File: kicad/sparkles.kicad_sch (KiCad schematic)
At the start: 70 parts

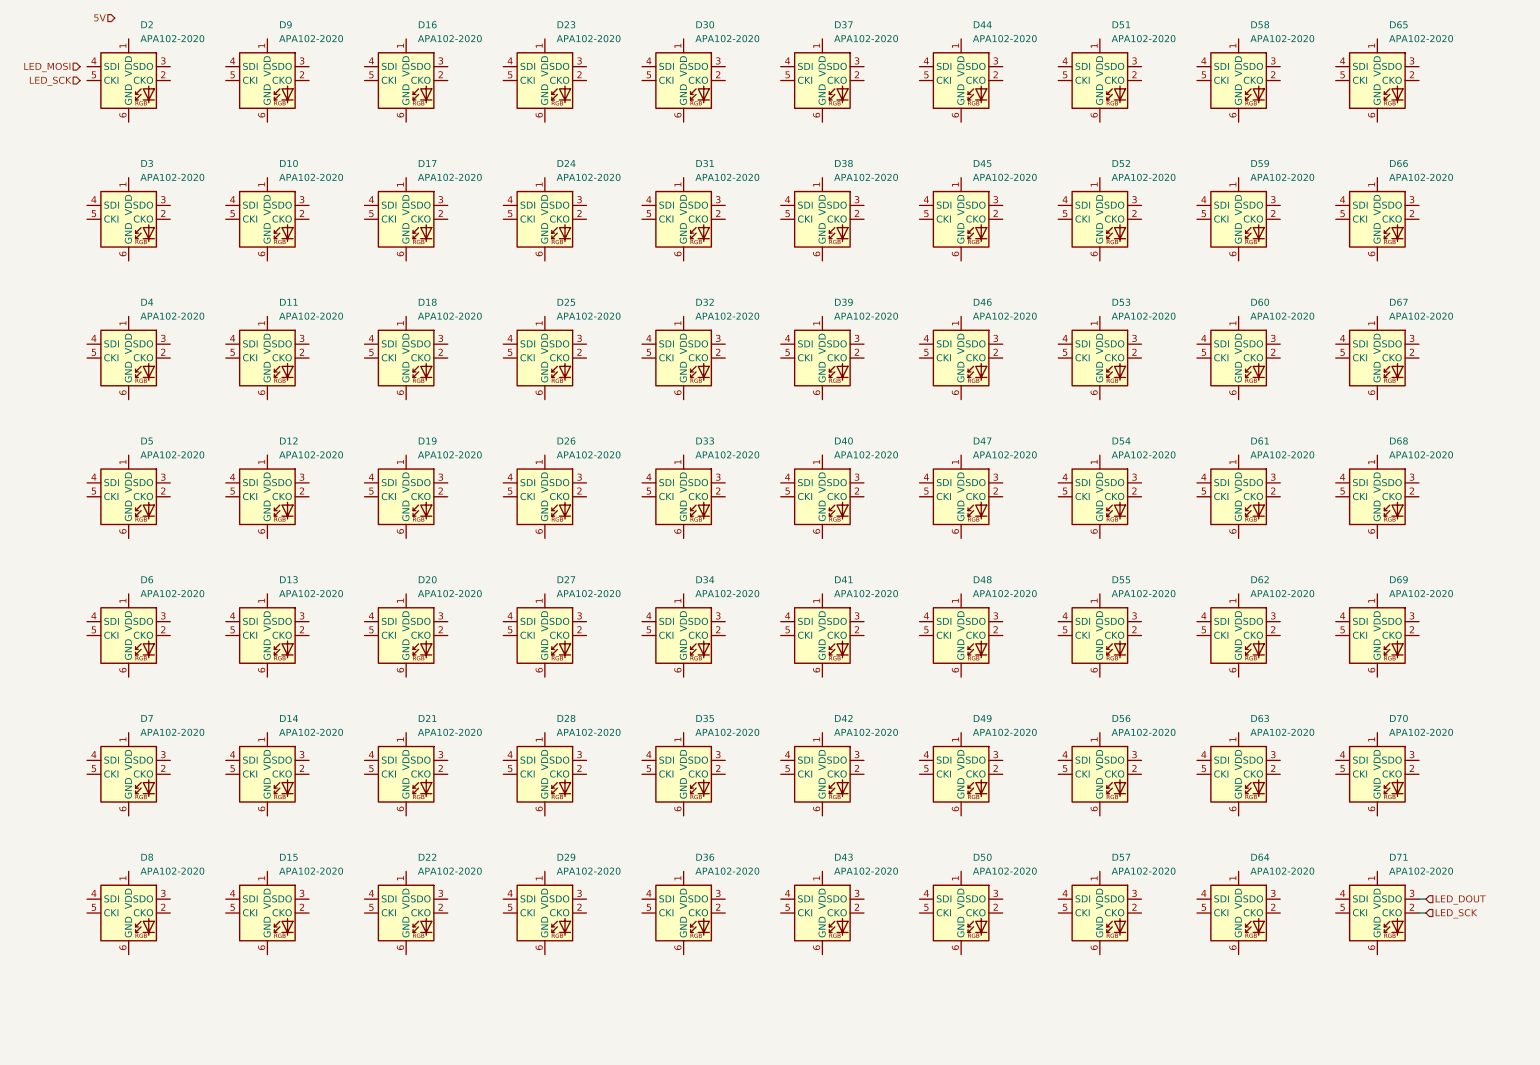
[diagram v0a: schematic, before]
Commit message: updates
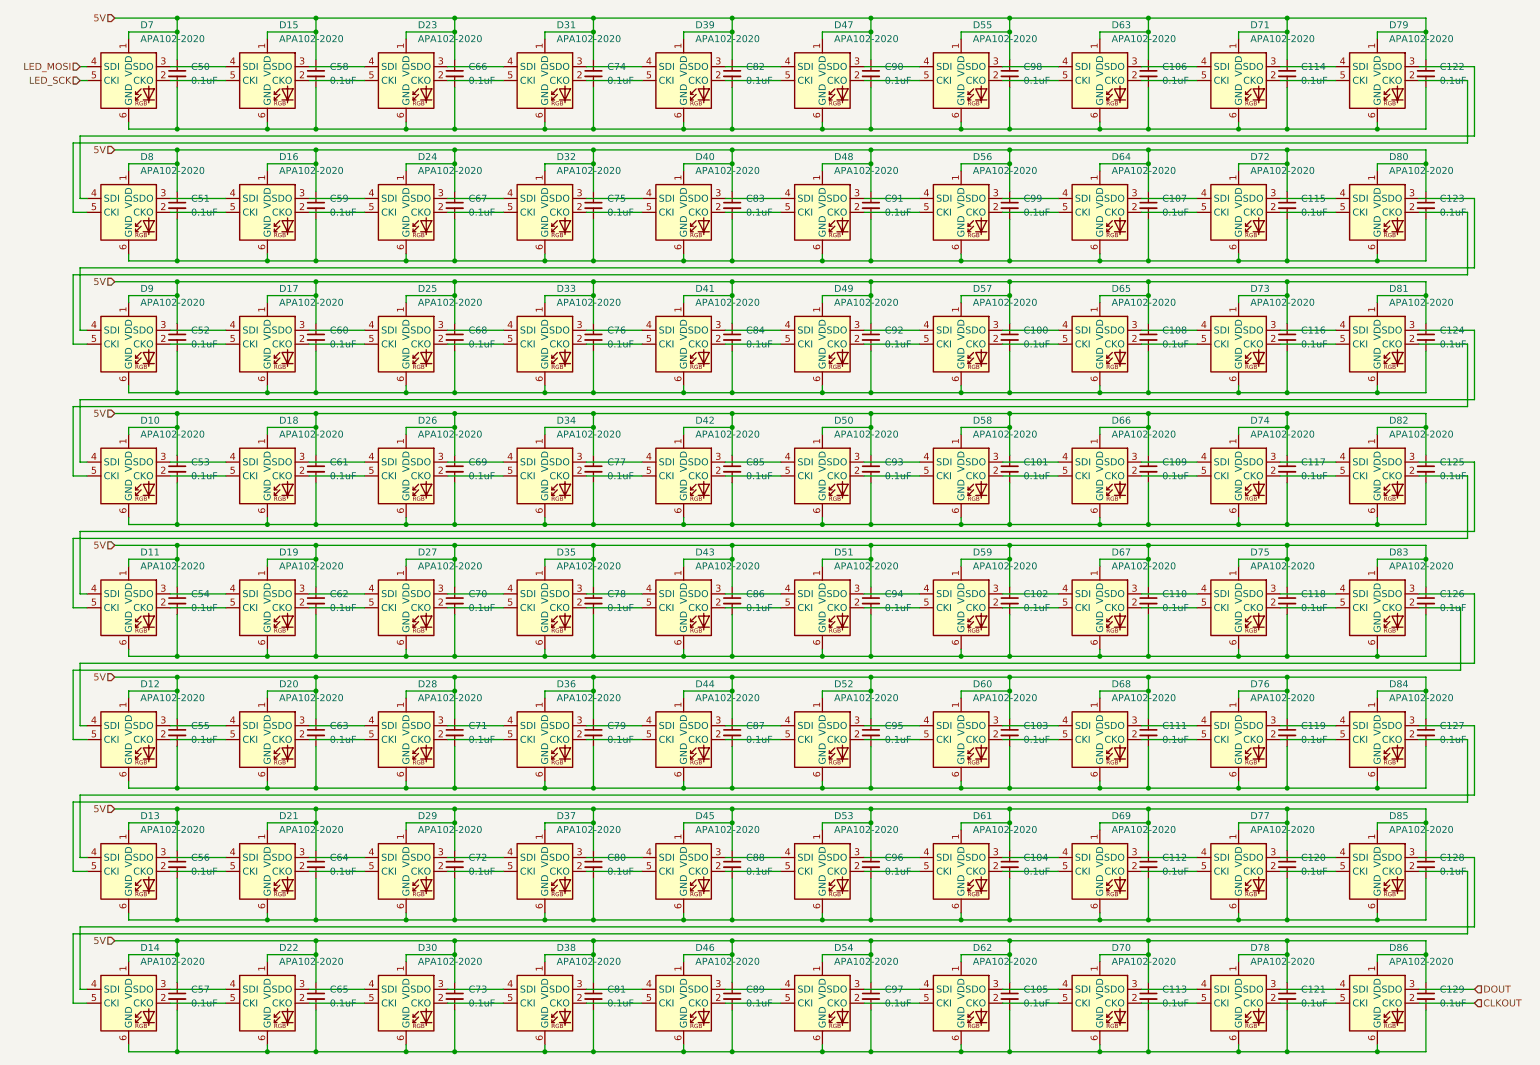
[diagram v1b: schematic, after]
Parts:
- removed D15, D3, D31, D39, D4, D47, D5, D55, D6, D63, D7, D71: APA102-2020, LED_SMD:LED-APA102-2020, symbol LED:APA102-2020
- added C100, C101, C102, C103, C104, C105, C106, C107, C108, C109, C110, C111, C112, C113, C114, C115, C116, C117, C118, C119, C120, C121, C122, C123, C124, C125, C126, C127, C128, C129, C50, C51, C52, C53, C54, C55, C56, C57, C58, C59, C60, C61, C62, C63, C64, C65, C66, C67, C68, C69, C70, C71, C72, C73, C74, C75, C76, C77, C78, C79, C80, C81, C82, C83, C84, C85, C86, C87, C88, C89, C90, C91, C92, C93, C94, C95, C96, C97, C98, C99: 0.1uF, symbol Device:C_Small
- added D16, D30, D37, D44, D51, D58, D65, D72, D73, D74, D75, D76, D77, D78, D80, D81, D82, D83, D84, D85, D86, D9: APA102-2020, LED_SMD:LED-APA102-2020, symbol LED:APA102-2020
- renumbered D9 to D15, D16 to D23, D23 to D31, D30 to D39, D37 to D47, D44 to D55, D51 to D63, D2 to D7, D58 to D71, D65 to D79
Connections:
- net 5V: now also D10.1 (VDD), D11.1 (VDD), D12.1 (VDD), D13.1 (VDD), D14.1 (VDD), D15.1 (VDD), D17.1 (VDD), D18.1 (VDD), D19.1 (VDD), D20.1 (VDD), D21.1 (VDD), D22.1 (VDD), D23.1 (VDD), D24.1 (VDD), D25.1 (VDD), D26.1 (VDD), D27.1 (VDD), D28.1 (VDD), D29.1 (VDD), D31.1 (VDD), D32.1 (VDD), D33.1 (VDD), D34.1 (VDD), D35.1 (VDD), D36.1 (VDD), D38.1 (VDD), D39.1 (VDD), D40.1 (VDD), D41.1 (VDD), D42.1 (VDD), D43.1 (VDD), D45.1 (VDD), D46.1 (VDD), D47.1 (VDD), D48.1 (VDD), D49.1 (VDD), D50.1 (VDD), D52.1 (VDD), D53.1 (VDD), D54.1 (VDD), D55.1 (VDD), D56.1 (VDD), D57.1 (VDD), D59.1 (VDD), D60.1 (VDD), D61.1 (VDD), D62.1 (VDD), D63.1 (VDD), D64.1 (VDD), D66.1 (VDD), D67.1 (VDD), D68.1 (VDD), D69.1 (VDD), D7.1 (VDD), D70.1 (VDD), D71.1 (VDD), D79.1 (VDD), D8.1 (VDD), C100.1, C101.1, C102.1, C103.1, C104.1, C105.1, C106.1, C107.1, C108.1, C109.1, C110.1, C111.1, C112.1, C113.1, C114.1, C115.1, C116.1, C117.1, C118.1, C119.1, C120.1, C121.1, C122.1, C123.1, C124.1, C125.1, C126.1, C127.1, C128.1, C129.1, C50.1, C51.1, C52.1, C53.1, C54.1, C55.1, C56.1, C57.1, C58.1, C59.1, C60.1, C61.1, C62.1, C63.1, C64.1, C65.1, C66.1, C67.1, C68.1, C69.1, C70.1, C71.1, C72.1, C73.1, C74.1, C75.1, C76.1, C77.1, C78.1, C79.1, C80.1, C81.1, C82.1, C83.1, C84.1, C85.1, C86.1, C87.1, C88.1, C89.1, C90.1, C91.1, C92.1, C93.1, C94.1, C95.1, C96.1, C97.1, C98.1, C99.1, D16.1 (VDD), D30.1 (VDD), D37.1 (VDD), D44.1 (VDD), D51.1 (VDD), D58.1 (VDD), D65.1 (VDD), D72.1 (VDD), D73.1 (VDD), D74.1 (VDD), D75.1 (VDD), D76.1 (VDD), D77.1 (VDD), D78.1 (VDD), D80.1 (VDD), D81.1 (VDD), D82.1 (VDD), D83.1 (VDD), D84.1 (VDD), D85.1 (VDD), D86.1 (VDD), D9.1 (VDD)
- net LED_MOSI: now also D7.4 (SDI)
- net LED_SCK: now also D7.5 (CKI)
- net at D32.2 (CKO): now also D40.5 (CKI)
- net at D32.3 (SDO): now also D40.4 (SDI)
- net at D32.4 (SDI): now also D24.3 (SDO)
- net at D32.5 (CKI): now also D24.2 (CKO)
- net at D32.6 (GND): now also D24.6 (GND), D40.6 (GND), D48.6 (GND), D56.6 (GND), D64.6 (GND), D8.6 (GND), C107.2, C115.2, C123.2, C51.2, C59.2, C67.2, C75.2, C83.2, C91.2, C99.2, D16.6 (GND), D72.6 (GND), D80.6 (GND)
- net at D21.2 (CKO): now also D29.5 (CKI)
- net at D21.3 (SDO): now also D29.4 (SDI)
- net at D21.4 (SDI): now also D13.3 (SDO)
- net at D21.5 (CKI): now also D13.2 (CKO)
- net at D21.6 (GND): now also D13.6 (GND), D29.6 (GND), D45.6 (GND), D53.6 (GND), D61.6 (GND), D69.6 (GND), C104.2, C112.2, C120.2, C128.2, C56.2, C64.2, C72.2, C80.2, C88.2, C96.2, D37.6 (GND), D77.6 (GND), D85.6 (GND)
- net at D34.2 (CKO): now also D42.5 (CKI)
- net at D34.3 (SDO): now also D42.4 (SDI)
- net at D34.4 (SDI): now also D26.3 (SDO)
- net at D34.5 (CKI): now also D26.2 (CKO)
- net at D34.6 (GND): now also D10.6 (GND), D18.6 (GND), D26.6 (GND), D42.6 (GND), D50.6 (GND), D66.6 (GND), C101.2, C109.2, C117.2, C125.2, C53.2, C61.2, C69.2, C77.2, C85.2, C93.2, D58.6 (GND), D74.6 (GND), D82.6 (GND)
- net at D48.2 (CKO): now also D56.5 (CKI)
- net at D48.3 (SDO): now also D56.4 (SDI)
- net at D48.4 (SDI): now also D40.3 (SDO)
- net at D48.5 (CKI): now also D40.2 (CKO)
- net at D64.2 (CKO): now also D72.5 (CKI)
- net at D64.3 (SDO): now also D72.4 (SDI)
- net at D64.4 (SDI): now also D56.3 (SDO)
- net at D64.5 (CKI): now also D56.2 (CKO)
- net at D47.2 (CKO): now also D55.5 (CKI)
- net at D47.3 (SDO): now also D55.4 (SDI)
- net at D47.4 (SDI): now also D39.3 (SDO)
- net at D47.5 (CKI): now also D39.2 (CKO)
- net at D47.6 (GND): now also D15.6 (GND), D23.6 (GND), D31.6 (GND), D39.6 (GND), D55.6 (GND), D63.6 (GND), D7.6 (GND), D71.6 (GND), D79.6 (GND), C106.2, C114.2, C122.2, C50.2, C58.2, C66.2, C74.2, C82.2, C90.2, C98.2
- net at D39.4 (SDI): now also D31.3 (SDO)
- net at D39.5 (CKI): now also D31.2 (CKO)
- net at D36.2 (CKO): now also D44.5 (CKI)
- net at D36.3 (SDO): now also D44.4 (SDI)
- net at D36.4 (SDI): now also D28.3 (SDO)
- net at D36.5 (CKI): now also D28.2 (CKO)
- net at D36.6 (GND): now also D12.6 (GND), D20.6 (GND), D28.6 (GND), D52.6 (GND), D60.6 (GND), D68.6 (GND), C103.2, C111.2, C119.2, C127.2, C55.2, C63.2, C71.2, C79.2, C87.2, C95.2, D44.6 (GND), D76.6 (GND), D84.6 (GND)
- net at D11.2 (CKO): now also D19.5 (CKI)
- net at D11.3 (SDO): now also D19.4 (SDI)
- net at D11.4 (SDI): now also D82.3 (SDO)
- net at D11.5 (CKI): now also D82.2 (CKO)
- net at D11.6 (GND): now also D19.6 (GND), D27.6 (GND), D35.6 (GND), D43.6 (GND), D59.6 (GND), D67.6 (GND), C102.2, C110.2, C118.2, C126.2, C54.2, C62.2, C70.2, C78.2, C86.2, C94.2, D51.6 (GND), D75.6 (GND), D83.6 (GND)
- net at D38.2 (CKO): now also D46.5 (CKI)
- net at D38.3 (SDO): now also D46.4 (SDI)
- net at D38.4 (SDI): now also D30.3 (SDO)
- net at D38.5 (CKI): now also D30.2 (CKO)
- net at D38.6 (GND): now also D14.6 (GND), D22.6 (GND), D46.6 (GND), D54.6 (GND), D62.6 (GND), D70.6 (GND), C105.2, C113.2, C121.2, C129.2, C57.2, C65.2, C73.2, C81.2, C89.2, C97.2, D30.6 (GND), D78.6 (GND), D86.6 (GND)
- net at D61.2 (CKO): now also D69.5 (CKI)
- net at D61.3 (SDO): now also D69.4 (SDI)
- net at D61.4 (SDI): now also D53.3 (SDO)
- net at D61.5 (CKI): now also D53.2 (CKO)
- net at D46.2 (CKO): now also D54.5 (CKI)
- net at D46.3 (SDO): now also D54.4 (SDI)
- net at D23.2 (CKO): now also D31.5 (CKI)
- net at D23.3 (SDO): now also D31.4 (SDI)
- net at D23.4 (SDI): now also D15.3 (SDO)
- net at D23.5 (CKI): now also D15.2 (CKO)
- net at D18.2 (CKO): now also D26.5 (CKI)
- net at D18.3 (SDO): now also D26.4 (SDI)
- net at D18.4 (SDI): now also D10.3 (SDO)
- net at D18.5 (CKI): now also D10.2 (CKO)
- net at D67.2 (CKO): now also D75.5 (CKI)
- net at D67.3 (SDO): now also D75.4 (SDI)
- net at D67.4 (SDI): now also D59.3 (SDO)
- net at D67.5 (CKI): now also D59.2 (CKO)
- net at D62.2 (CKO): now also D70.5 (CKI)
- net at D62.3 (SDO): now also D70.4 (SDI)
- net at D62.4 (SDI): now also D54.3 (SDO)
- net at D62.5 (CKI): now also D54.2 (CKO)
- net at D28.4 (SDI): now also D20.3 (SDO)
- net at D28.5 (CKI): now also D20.2 (CKO)
- net at D29.2 (CKO): now also D37.5 (CKI)
- net at D29.3 (SDO): now also D37.4 (SDI)
- net at D25.2 (CKO): now also D33.5 (CKI)
- net at D25.3 (SDO): now also D33.4 (SDI)
- net at D25.4 (SDI): now also D17.3 (SDO)
- net at D25.5 (CKI): now also D17.2 (CKO)
- net at D25.6 (GND): now also D17.6 (GND), D33.6 (GND), D41.6 (GND), D49.6 (GND), D57.6 (GND), C100.2, C108.2, C116.2, C124.2, C52.2, C60.2, C68.2, C76.2, C84.2, C92.2, D65.6 (GND), D73.6 (GND), D81.6 (GND), D9.6 (GND)
- net at D24.4 (SDI): now also D16.3 (SDO)
- net at D24.5 (CKI): now also D16.2 (CKO)
- net at D52.2 (CKO): now also D60.5 (CKI)
- net at D52.3 (SDO): now also D60.4 (SDI)
- net at D52.4 (SDI): now also D44.3 (SDO)
- net at D52.5 (CKI): now also D44.2 (CKO)
- net at D60.2 (CKO): now also D68.5 (CKI)
- net at D60.3 (SDO): now also D68.4 (SDI)
- net at D42.2 (CKO): now also D50.5 (CKI)
- net at D42.3 (SDO): now also D50.4 (SDI)
- net at D15.4 (SDI): now also D7.3 (SDO)
- net at D15.5 (CKI): now also D7.2 (CKO)
- net at D79.2 (CKO): now also D8.5 (CKI)
- net at D79.3 (SDO): now also D8.4 (SDI)
- net at D79.4 (SDI): now also D71.3 (SDO)
- net at D79.5 (CKI): now also D71.2 (CKO)
- net at D66.2 (CKO): now also D74.5 (CKI)
- net at D66.3 (SDO): now also D74.4 (SDI)
- net at D66.4 (SDI): now also D58.3 (SDO)
- net at D66.5 (CKI): now also D58.2 (CKO)
- net at D20.4 (SDI): now also D12.3 (SDO)
- net at D20.5 (CKI): now also D12.2 (CKO)
- net at D63.2 (CKO): now also D71.5 (CKI)
- net at D63.3 (SDO): now also D71.4 (SDI)
- net at D63.4 (SDI): now also D55.3 (SDO)
- net at D63.5 (CKI): now also D55.2 (CKO)
- net at D35.2 (CKO): now also D43.5 (CKI)
- net at D35.3 (SDO): now also D43.4 (SDI)
- net at D35.4 (SDI): now also D27.3 (SDO)
- net at D35.5 (CKI): now also D27.2 (CKO)
- net at D14.2 (CKO): now also D22.5 (CKI)
- net at D14.3 (SDO): now also D22.4 (SDI)
- net at D14.4 (SDI): now also D85.3 (SDO)
- net at D14.5 (CKI): now also D85.2 (CKO)
- net at D27.4 (SDI): now also D19.3 (SDO)
- net at D27.5 (CKI): now also D19.2 (CKO)
- net at D12.4 (SDI): now also D83.3 (SDO)
- net at D12.5 (CKI): now also D83.2 (CKO)
- net at D50.2 (CKO): now also D58.5 (CKI)
- net at D50.3 (SDO): now also D58.4 (SDI)
- net at D13.4 (SDI): now also D84.3 (SDO)
- net at D13.5 (CKI): now also D84.2 (CKO)
- net at D69.2 (CKO): now also D77.5 (CKI)
- net at D69.3 (SDO): now also D77.4 (SDI)
- net at D70.2 (CKO): now also D78.5 (CKI)
- net at D70.3 (SDO): now also D78.4 (SDI)
- net at D43.2 (CKO): now also D51.5 (CKI)
- net at D43.3 (SDO): now also D51.4 (SDI)
- net at D8.2 (CKO): now also D16.5 (CKI)
- net at D8.3 (SDO): now also D16.4 (SDI)
- net at D10.4 (SDI): now also D81.3 (SDO)
- net at D10.5 (CKI): now also D81.2 (CKO)
- net at D41.2 (CKO): now also D49.5 (CKI)
- net at D41.3 (SDO): now also D49.4 (SDI)
- net at D41.4 (SDI): now also D33.3 (SDO)
- net at D41.5 (CKI): now also D33.2 (CKO)
- net at D17.4 (SDI): now also D9.3 (SDO)
- net at D17.5 (CKI): now also D9.2 (CKO)
- net at D57.2 (CKO): now also D65.5 (CKI)
- net at D57.3 (SDO): now also D65.4 (SDI)
- net at D57.4 (SDI): now also D49.3 (SDO)
- net at D57.5 (CKI): now also D49.2 (CKO)
- net at D22.2 (CKO): now also D30.5 (CKI)
- net at D22.3 (SDO): now also D30.4 (SDI)
- net at D59.4 (SDI): now also D51.3 (SDO)
- net at D59.5 (CKI): now also D51.2 (CKO)
- net at D53.4 (SDI): now also D45.3 (SDO)
- net at D53.5 (CKI): now also D45.2 (CKO)
- net at D68.2 (CKO): now also D76.5 (CKI)
- net at D68.3 (SDO): now also D76.4 (SDI)
- net at D45.4 (SDI): now also D37.3 (SDO)
- net at D45.5 (CKI): now also D37.2 (CKO)
- new net: D77.3 (SDO), D85.4 (SDI)
- new net: D77.2 (CKO), D85.5 (CKI)
- new net: D74.3 (SDO), D82.4 (SDI)
- new net: D74.2 (CKO), D82.5 (CKI)
- new net: D80.3 (SDO), D9.4 (SDI)
- new net: D80.2 (CKO), D9.5 (CKI)
- new net: D72.3 (SDO), D80.4 (SDI)
- new net: D72.2 (CKO), D80.5 (CKI)
- new net: D75.3 (SDO), D83.4 (SDI)
- new net: D75.2 (CKO), D83.5 (CKI)
- new net: D65.2 (CKO), D73.5 (CKI)
- new net: D65.3 (SDO), D73.4 (SDI)
- new net: D73.3 (SDO), D81.4 (SDI)
- new net: D73.2 (CKO), D81.5 (CKI)
- new net: D76.3 (SDO), D84.4 (SDI)
- new net: D76.2 (CKO), D84.5 (CKI)
- new net: D78.2 (CKO), D86.5 (CKI)
- new net: D78.3 (SDO), D86.4 (SDI)
- new net CLKOUT: D86.2 (CKO)
- new net DOUT: D86.3 (SDO)
